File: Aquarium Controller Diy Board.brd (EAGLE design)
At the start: 126.9 x 90.2 mm, 46 parts

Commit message: 2
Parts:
- C1: device resistor:C0805K -> rcl:C0805K
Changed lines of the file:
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@@
 <layer number="54" name="bGND_GNDA" color="1" fill="9" visible="no" active="no"/>
 <layer number="56" name="wert" color="7" fill="1" visible="no" active="yes"/>
+<layer number="90" name="Modules" color="5" fill="1" visible="no" active="no"/>
 <layer number="91" name="Nets" color="2" fill="1" visible="no" active="no"/>
 <layer number="92" name="Busses" color="1" fill="1" visible="no" active="no"/>
@@
 <element name="R14" library="rcl" package="R0805" value="1K" x="100.33" y="36.83" rot="MR0"/>
 <element name="R15" library="rcl" package="R0805" value="10K" x="100.33" y="39.37" rot="MR180"/>
-<element name="C1" library="resistor" package="C0805K" value=".1uF" x="99.06" y="34.29" rot="MR0"/>
+<element name="C1" library="rcl" package="C0805K" value=".1uF" x="99.06" y="34.29" rot="MR0"/>
 <element name="C2" library="resistor" package="C0805K" value=".1uF" x="93.98" y="34.29" rot="MR180"/>
 <element name="R16" library="rcl" package="R0805" value="10K" x="92.71" y="62.23" rot="MR0"/>

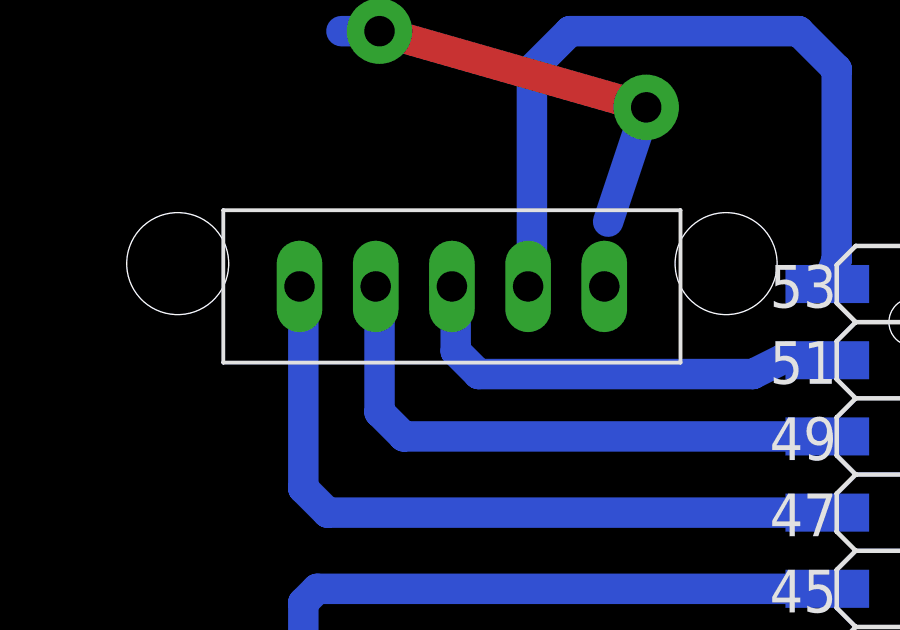
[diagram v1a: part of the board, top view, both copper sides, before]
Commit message: 4
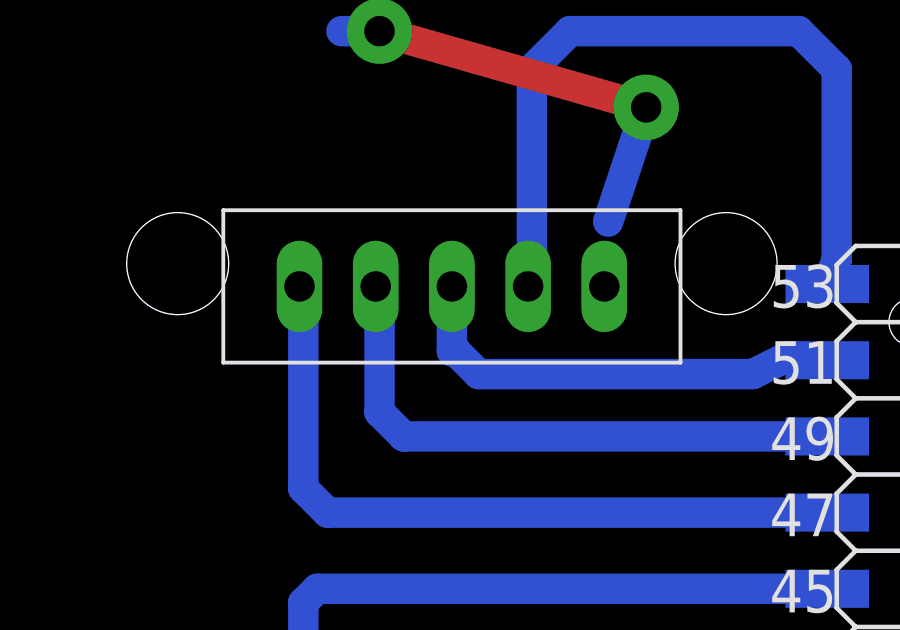
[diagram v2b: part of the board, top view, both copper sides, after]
